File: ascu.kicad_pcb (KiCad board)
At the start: 2 copper layers, 80.6 x 42.7 mm, 91 parts, among them IC1 ATTINY25-SS, P1 B-, P10 CONN_01X01, P11 CONN_01X01, P12 CONN_01X01, P13 CONN_01X01, P14 CONN_01X01, P15 CONN_01X01, P16 CONN_01X01, P17 CONN_01X01, P18 CONN_01X01, P19 CONN_01X01, P2 B+S+, P20 CONN_01X01, P21 CONN_01X01, P22 CONN_01X01, P23 CONN_01X01, P24 CONN_01X01, P25 CONN_01X01, P26 CONN_01X01, P27 CONN_01X01, P28 CONN_01X01, P29 CONN_01X01, P3 S-, P30 CONN_01X01, P31 CONN_01X01, P32 CONN_01X01, P33 CONN_01X01, P34 CONN_01X01, P35 CONN_01X01, P37 Otwór, P38 Otwór, P39 Otwór, P4 CONN_01X01, P40 Otwór, P41 Lut, P42 Lut, P43 Lut, P44 Lut, P45 Lut, P46 Lut, P47 Lut, P48 Lut, P49 Lut, P5 CONN_01X01, P50 Lut, P51 Lut, P52 Lut, P53 Lut, P54 Lut, P55 Lut, P56 Lut, P6 CONN_01X01, P7 CONN_01X01, P8 CONN_01X01, P9 CONN_01X01, Q1 PSMN1R2, Q2 PSMN1R2, SW1 DETECT, SW3 TRIGGER, U1 SPX3819, U2 MIC4605, U3 TLP291

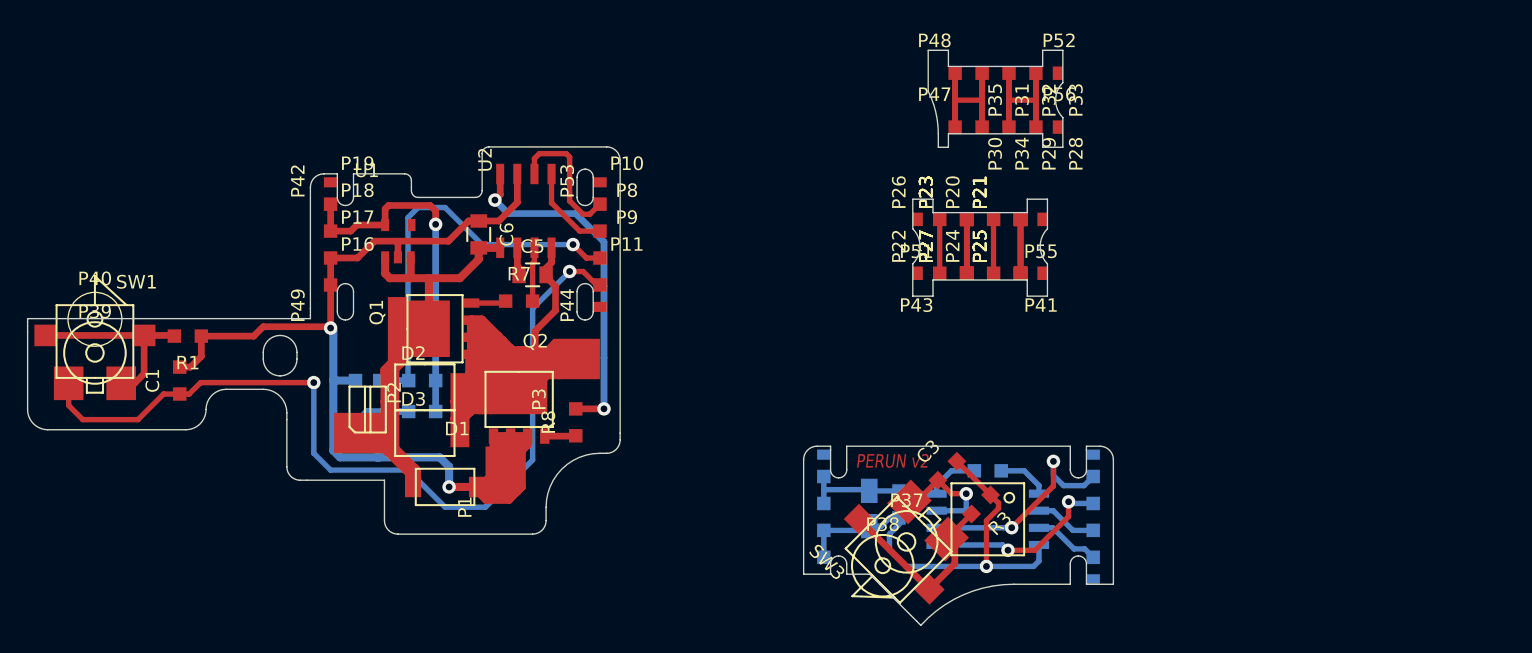
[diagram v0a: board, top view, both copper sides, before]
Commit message: Test
test
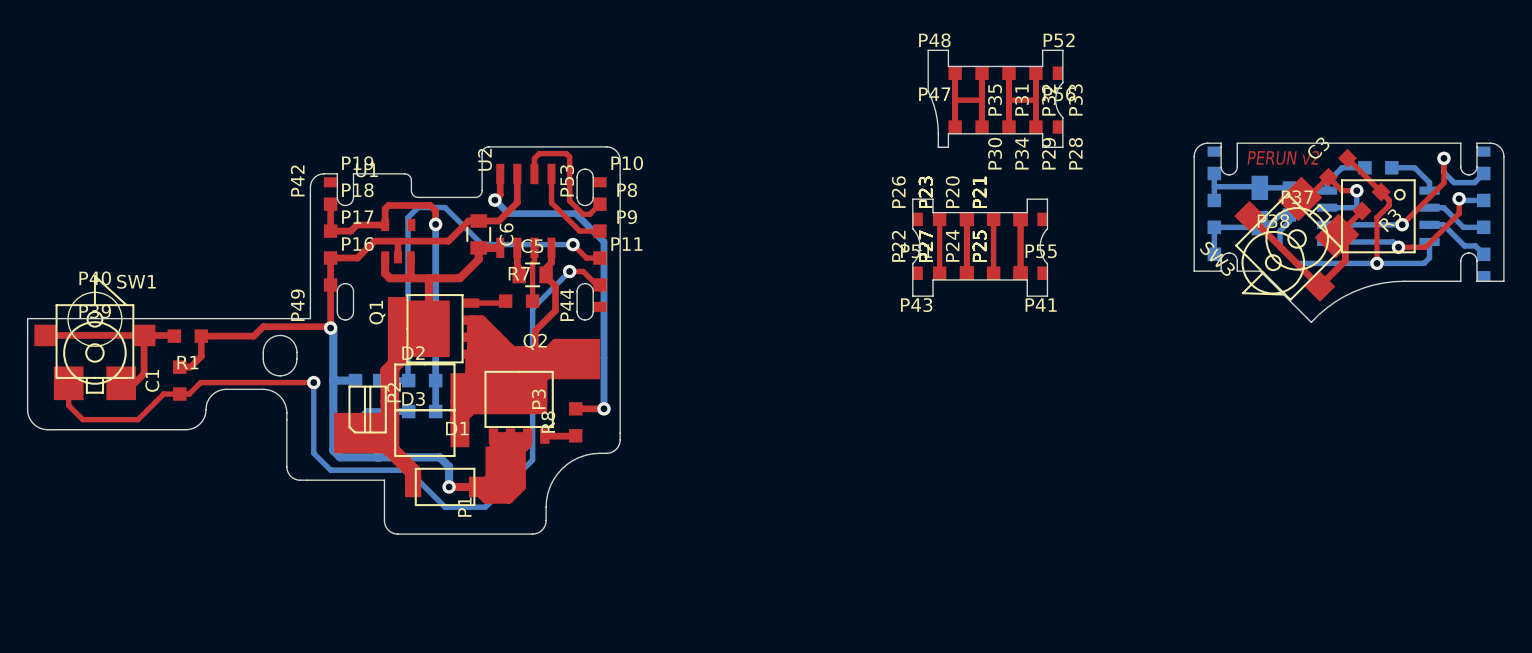
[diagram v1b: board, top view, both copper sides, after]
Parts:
- moved C2 36.7 mm to (200.5, 73.1)
- moved C3 36.7 mm to (206.3, 70.3)
- moved C4 36.7 mm to (202.7, 72.8)
- moved IC1 36.7 mm to (209.3, 73.9)
- moved P12 36.7 mm to (197.1, 74.7)
- moved P13 36.7 mm to (197.1, 76.7)
- moved P14 36.7 mm to (197.1, 70.7)
- moved P15 36.7 mm to (197.1, 72.7)
- moved P37 36.7 mm to (203.3, 75.6)
- moved P38 36.7 mm to (201.5, 77.3)
- moved P4 36.7 mm to (217.1, 72.7)
- moved P45 36.7 mm to (197.1, 78.3)
- moved P46 36.7 mm to (197.1, 69.1)
- moved P5 36.7 mm to (217.1, 74.7)
- moved P50 36.7 mm to (217.1, 69.1)
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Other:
- board size 80.6 x 42.7 mm -> 109.6 x 35.9 mm

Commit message: Poprawki
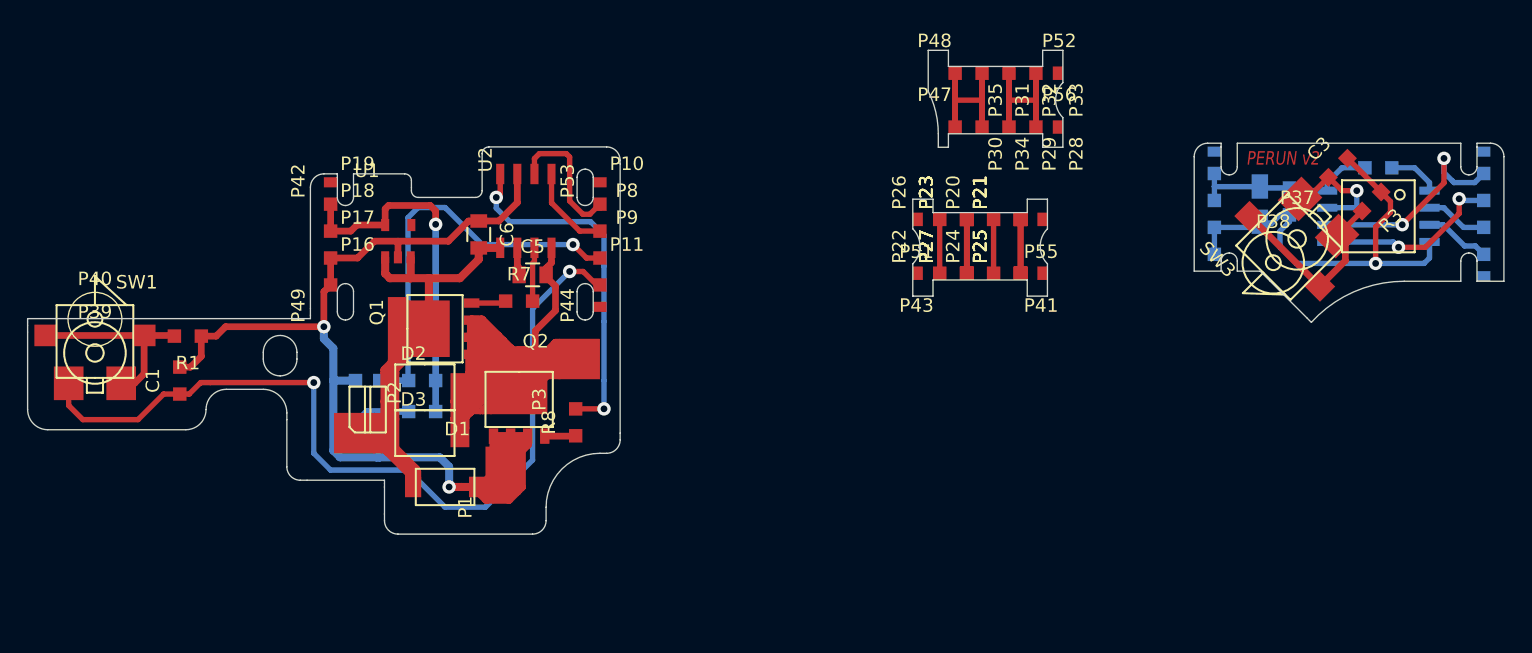
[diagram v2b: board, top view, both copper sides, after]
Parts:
- moved C2 0.10 mm to (200.5, 73.0)
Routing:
- net LO: track 26.0 -> 26.5 mm
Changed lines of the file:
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@@
     (links 93)
     (no_connects 0)
-    (area 108.899999 58.4 198.783334 110.600001)
+    (area 108.899999 58.4 227.783334 97.550001)
     (thickness 1)
     (drawings 181)
-    (tracks 475)
+    (tracks 478)
     (zones 0)
     (modules 91)
@@
   )
   (module Capacitors_Tantalum_SMD:TantalC_SizeA_EIA-3216_Reflow (layer B.Cu)
-    (at 200.5 73.1 270)
+    (at 200.5 73 270)
     (descr "Tantal Cap. , Size A, EIA-3216, Reflow")
     (tags "Tantal Capacitor Size-A EIA-3216 reflow")
@@
   (gr_line (start 128 81) (end 128 78.5) (angle 90) (layer Margin) (width 0.2))
   (gr_line (start 130 81) (end 128 81) (angle 90) (layer Margin) (width 0.2))
+  (segment (start 131 82.1) (end 131 83) (width 0.6) (layer B.Cu) (net 1))
+  (via (at 131 82.1) (size 1) (drill 0.5) (layers F.Cu B.Cu) (net 1))
+  (segment (start 131.7 83.7) (end 131.7 86.1) (width 0.6) (layer B.Cu) (net 1))
+  (segment (start 131 83) (end 131.7 83.7) (width 0.6) (layer B.Cu) (net 1))
+  (segment (start 131 82.1) (end 131 79.5) (width 0.5) (layer F.Cu) (net 1))
+  (segment (start 123 82.8) (end 123.7 82.1) (width 0.5) (layer F.Cu) (net 1))
+  (segment (start 123.7 82.1) (end 131 82.1) (width 0.5) (layer F.Cu) (net 1))
+  (segment (start 121.9 82.8) (end 123 82.8) (width 0.5) (layer F.Cu) (net 1) (status 400000))
+  (segment (start 131 79.5) (end 131.5 79) (width 0.5) (layer F.Cu) (net 1) (status 800000))
   (segment (start 120.3 85.1) (end 121.1 85.1) (width 0.5) (layer F.Cu) (net 1))
+  (segment (start 121.1 85.1) (end 121.9 84.3) (width 0.5) (layer F.Cu) (net 1))
   (segment (start 121.9 84.3) (end 121.9 82.8) (width 0.5) (layer F.Cu) (net 1))
-  (segment (start 121.1 85.1) (end 121.9 84.3) (width 0.5) (layer F.Cu) (net 1))
-  (segment (start 121.9 82.8) (end 125.8 82.8) (width 0.5) (layer F.Cu) (net 1))
-  (segment (start 131.4 82.1) (end 131.5 82.2) (width 0.5) (layer F.Cu) (net 1))
-  (segment (start 126.5 82.1) (end 131.4 82.1) (width 0.5) (layer F.Cu) (net 1))
-  (segment (start 125.8 82.8) (end 126.5 82.1) (width 0.5) (layer F.Cu) (net 1))
   (segment (start 135.15 90.4) (end 135.15 91.8) (width 0.6) (layer B.Cu) (net 1))
   (segment (start 135.15 91.8) (end 134.9 91.8) (width 0.6) (layer B.Cu) (net 1))
@@
   (segment (start 131.7 86.1) (end 131.9 86.1) (width 0.6) (layer B.Cu) (net 1))
   (segment (start 131.9 86.1) (end 131.7 86.1) (width 0.6) (layer B.Cu) (net 1))
-  (segment (start 131.5 82.2) (end 131.5 82.25) (width 0.6) (layer F.Cu) (net 1))
-  (segment (start 131.5 79) (end 131.5 82.25) (width 0.5) (layer F.Cu) (net 1))
-  (via (at 131.5 82.2) (size 1) (drill 0.5) (layers F.Cu B.Cu) (net 1))
-  (segment (start 131.7 86.1) (end 131.7 82.4) (width 0.6) (layer B.Cu) (net 1))
-  (segment (start 131.7 82.4) (end 131.5 82.2) (width 0.6) (layer B.Cu) (net 1))
   (segment (start 131.7 91.3) (end 131.7 86.1) (width 0.6) (layer B.Cu) (net 1))
+  (segment (start 132.2 91.8) (end 131.7 91.3) (width 0.6) (layer B.Cu) (net 1))
   (segment (start 134.9 91.8) (end 132.2 91.8) (width 0.6) (layer B.Cu) (net 1))
-  (segment (start 132.2 91.8) (end 131.7 91.3) (width 0.6) (layer B.Cu) (net 1))
   (segment (start 142.375 94) (end 143 94) (width 1.2) (layer F.Cu) (net 1))
   (segment (start 143 94) (end 144.5 92.5) (width 1.2) (layer F.Cu) (net 1))
@@
   (segment (start 203.656371 72.635913) (end 203.664087 72.635913) (width 0.4) (layer F.Cu) (net 11))
   (segment (start 205.5 71.995) (end 202.895 71.995) (width 0.4) (layer B.Cu) (net 12))
-  (segment (start 202.895 71.995) (end 202.7 71.8) (width 0.4) (layer B.Cu) (net 12))
   (segment (start 200.5 71.79) (end 202.69 71.79) (width 0.4) (layer B.Cu) (net 12))
-  (segment (start 202.69 71.79) (end 202.7 71.8) (width 0.4) (layer B.Cu) (net 12))
   (segment (start 197.125 71.7) (end 200.41 71.7) (width 0.4) (layer B.Cu) (net 12))
   (segment (start 200.41 71.7) (end 200.5 71.79) (width 0.4) (layer B.Cu) (net 12))
+  (segment (start 202.895 71.995) (end 202.7 71.8) (width 0.4) (layer B.Cu) (net 12))
+  (segment (start 202.69 71.79) (end 202.7 71.8) (width 0.4) (layer B.Cu) (net 12))
   (segment (start 197.125 72.725) (end 197.125 71.7) (width 0.4) (layer B.Cu) (net 12))
   (segment (start 197.125 71.7) (end 197.125 70.725) (width 0.4) (layer B.Cu) (net 12))
@@
   (segment (start 205.5 71.4) (end 205.5 71.995) (width 0.4) (layer B.Cu) (net 12))
   (segment (start 206.6 70.3) (end 205.5 71.4) (width 0.4) (layer B.Cu) (net 12))
-  (segment (start 209.507107 72.092893) (end 209.507107 72.107107) (width 0.4) (layer F.Cu) (net 13))
-  (segment (start 209.507107 72.107107) (end 210.1 72.7) (width 0.4) (layer F.Cu) (net 13))
-  (via (at 209.2 77.4) (size 1) (drill 0.5) (layers F.Cu B.Cu) (net 13))
-  (segment (start 209.2 74) (end 209.2 77.4) (width 0.4) (layer F.Cu) (net 13))
-  (segment (start 210.1 73.1) (end 209.2 74) (width 0.4) (layer F.Cu) (net 13))
-  (segment (start 210.1 72.7) (end 210.1 73.1) (width 0.4) (layer F.Cu) (net 13))
+  (segment (start 209.507107 72.092893) (end 209.507107 72.107107) (width 0.4) (layer F.Cu) (net 13) (status C00000))
+  (segment (start 209.507107 72.107107) (end 210.2 72.8) (width 0.4) (layer F.Cu) (net 13) (status 400000))
+  (segment (start 209.1 77.4) (end 209.2 77.4) (width 0.4) (layer B.Cu) (net 13))
+  (via (at 209.1 77.4) (size 1) (drill 0.5) (layers F.Cu B.Cu) (net 13))
+  (segment (start 209.1 74.7) (end 209.1 77.4) (width 0.4) (layer F.Cu) (net 13))
+  (segment (start 210.2 73.6) (end 209.1 74.7) (width 0.4) (layer F.Cu) (net 13))
+  (segment (start 210.2 72.8) (end 210.2 73.6) (width 0.4) (layer F.Cu) (net 13))
+  (segment (start 200.5 74.41) (end 201.39 74.41) (width 0.4) (layer B.Cu) (net 13))
+  (segment (start 201.39 74.41) (end 202 73.8) (width 0.4) (layer B.Cu) (net 13))
+  (segment (start 202 73.8) (end 202.7 73.8) (width 0.4) (layer B.Cu) (net 13))
+  (segment (start 197.125 74.725) (end 200.185 74.725) (width 0.4) (layer B.Cu) (net 13))
+  (segment (start 202.7 74.3) (end 202 75) (width 0.4) (layer B.Cu) (net 13))
+  (segment (start 202 75) (end 202 76.2) (width 0.4) (layer B.Cu) (net 13))
+  (segment (start 202 76.2) (end 203.2 77.4) (width 0.4) (layer B.Cu) (net 13))
+  (segment (start 203.2 77.4) (end 209.2 77.4) (width 0.4) (layer B.Cu) (net 13))
+  (segment (start 202.7 73.8) (end 202.7 74.3) (width 0.4) (layer B.Cu) (net 13))
+  (segment (start 200.185 74.725) (end 200.5 74.41) (width 0.4) (layer B.Cu) (net 13))
   (segment (start 209.507107 72.092893) (end 207.007107 69.592893) (width 0.4) (layer F.Cu) (net 13))
-  (segment (start 202.7 73.8) (end 202.7 74.3) (width 0.4) (layer B.Cu) (net 13))
-  (segment (start 202.7 74.3) (end 202 75) (width 0.4) (layer B.Cu) (net 13))
   (segment (start 213.1 77) (end 213.1 75.805) (width 0.4) (layer B.Cu) (net 13))
   (segment (start 212.7 77.4) (end 213.1 77) (width 0.4) (layer B.Cu) (net 13))
-  (segment (start 203.2 77.4) (end 209.2 77.4) (width 0.4) (layer B.Cu) (net 13))
   (segment (start 209.2 77.4) (end 212.7 77.4) (width 0.4) (layer B.Cu) (net 13))
-  (segment (start 202 76.2) (end 203.2 77.4) (width 0.4) (layer B.Cu) (net 13))
-  (segment (start 202 75) (end 202 76.2) (width 0.4) (layer B.Cu) (net 13))
-  (segment (start 200.5 74.41) (end 201.39 74.41) (width 0.4) (layer B.Cu) (net 13))
-  (segment (start 202 73.8) (end 202.7 73.8) (width 0.4) (layer B.Cu) (net 13))
-  (segment (start 201.39 74.41) (end 202 73.8) (width 0.4) (layer B.Cu) (net 13))
-  (segment (start 197.125 74.725) (end 200.185 74.725) (width 0.4) (layer B.Cu) (net 13))
-  (segment (start 200.185 74.725) (end 200.5 74.41) (width 0.4) (layer B.Cu) (net 13))
   (segment (start 197.125 76.725) (end 197.125 74.725) (width 0.4) (layer B.Cu) (net 13))
   (segment (start 213.1 73.265) (end 214.165 73.265) (width 0.4) (layer B.Cu) (net 14))
@@
   (segment (start 146.5 77.4) (end 146.5 80.2) (width 0.4) (layer F.Cu) (net 29))
   (segment (start 146.635 77.265) (end 146.5 77.4) (width 0.4) (layer F.Cu) (net 29))
-  (segment (start 149.7 88.2) (end 151.8 88.2) (width 0.5) (layer F.Cu) (net 30))
-  (segment (start 144.095 72.305) (end 144.095 70.76) (width 0.5) (layer F.Cu) (net 30))
-  (segment (start 143.7 72.7) (end 144.095 72.305) (width 0.5) (layer F.Cu) (net 30))
-  (via (at 143.7 72.7) (size 1) (drill 0.5) (layers F.Cu B.Cu) (net 30))
-  (segment (start 144.7 73.7) (end 143.7 72.7) (width 0.5) (layer B.Cu) (net 30))
-  (segment (start 149.7 73.7) (end 144.7 73.7) (width 0.5) (layer B.Cu) (net 30))
-  (segment (start 151.8 75.8) (end 149.7 73.7) (width 0.5) (layer B.Cu) (net 30))
-  (segment (start 151.8 79.1) (end 151.8 75.8) (width 0.5) (layer B.Cu) (net 30))
-  (segment (start 151.8 84.4) (end 151.8 79.1) (width 0.5) (layer B.Cu) (net 30))
-  (segment (start 151.8 88.2) (end 151.8 84.4) (width 0.5) (layer B.Cu) (net 30))
+  (segment (start 149.7 88.2) (end 151.8 88.2) (width 0.4) (layer F.Cu) (net 30) (status 400000))
+  (segment (start 144.095 72.205) (end 144.095 70.76) (width 0.4) (layer F.Cu) (net 30) (status 800000))
+  (segment (start 143.8 72.5) (end 144.095 72.205) (width 0.4) (layer F.Cu) (net 30))
+  (via (at 143.8 72.5) (size 1) (drill 0.5) (layers F.Cu B.Cu) (net 30))
+  (segment (start 143.8 73.3) (end 143.8 72.5) (width 0.4) (layer B.Cu) (net 30))
+  (segment (start 144.8 74.3) (end 143.8 73.3) (width 0.4) (layer B.Cu) (net 30))
+  (segment (start 150.8 74.3) (end 144.8 74.3) (width 0.4) (layer B.Cu) (net 30))
+  (segment (start 151.8 75.3) (end 150.8 74.3) (width 0.4) (layer B.Cu) (net 30))
+  (segment (start 151.8 77.6) (end 151.8 75.3) (width 0.4) (layer B.Cu) (net 30))
+  (segment (start 151.8 81.7) (end 151.8 77.6) (width 0.4) (layer B.Cu) (net 30))
+  (segment (start 151.8 86.1) (end 151.8 81.7) (width 0.4) (layer B.Cu) (net 30))
+  (segment (start 151.8 88.2) (end 151.8 86.1) (width 0.4) (layer B.Cu) (net 30))
   (via (at 151.8 88.2) (size 1) (drill 0.5) (layers F.Cu B.Cu) (net 30))
   (zone (net 0) (net_name "") (layer B.Paste) (hatch none 0.508)
